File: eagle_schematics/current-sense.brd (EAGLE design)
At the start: 76.2 x 46.7 mm, 19 parts, among them IC1 MCP601P

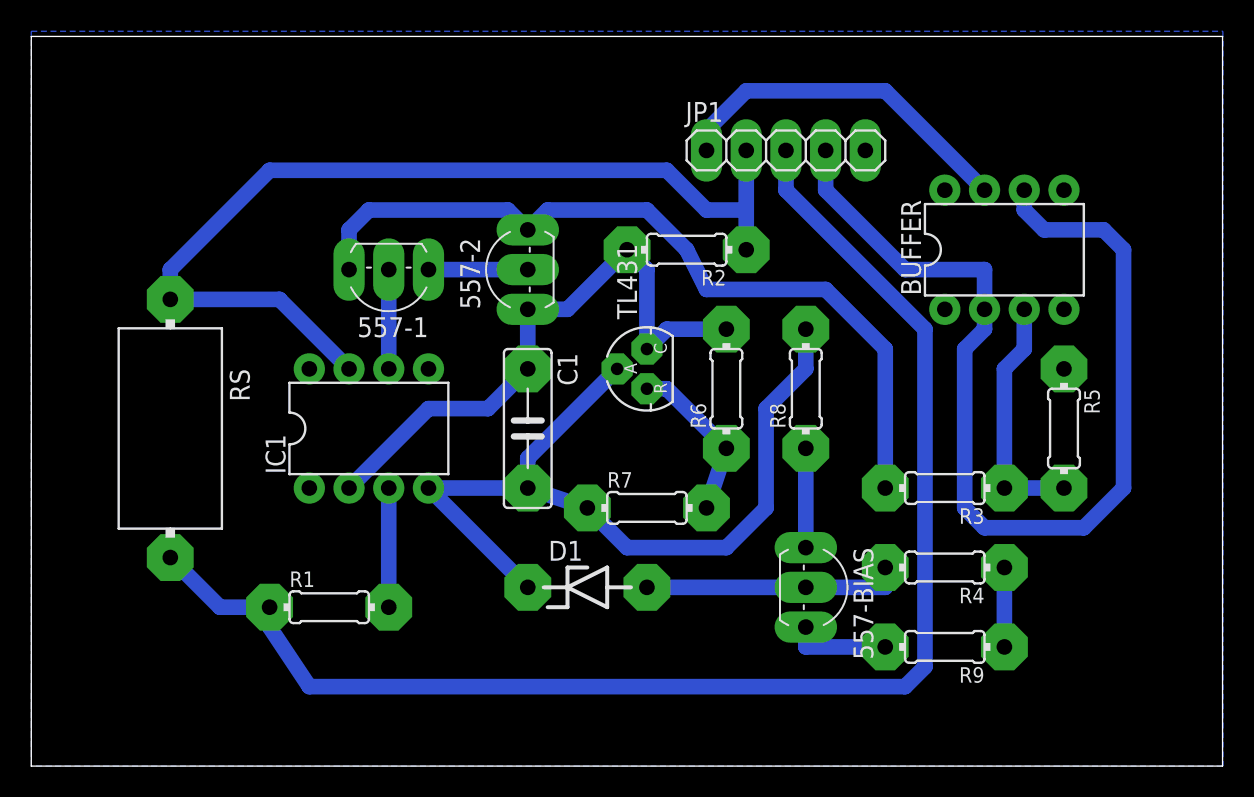
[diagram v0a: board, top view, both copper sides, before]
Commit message: mais esquemáticos
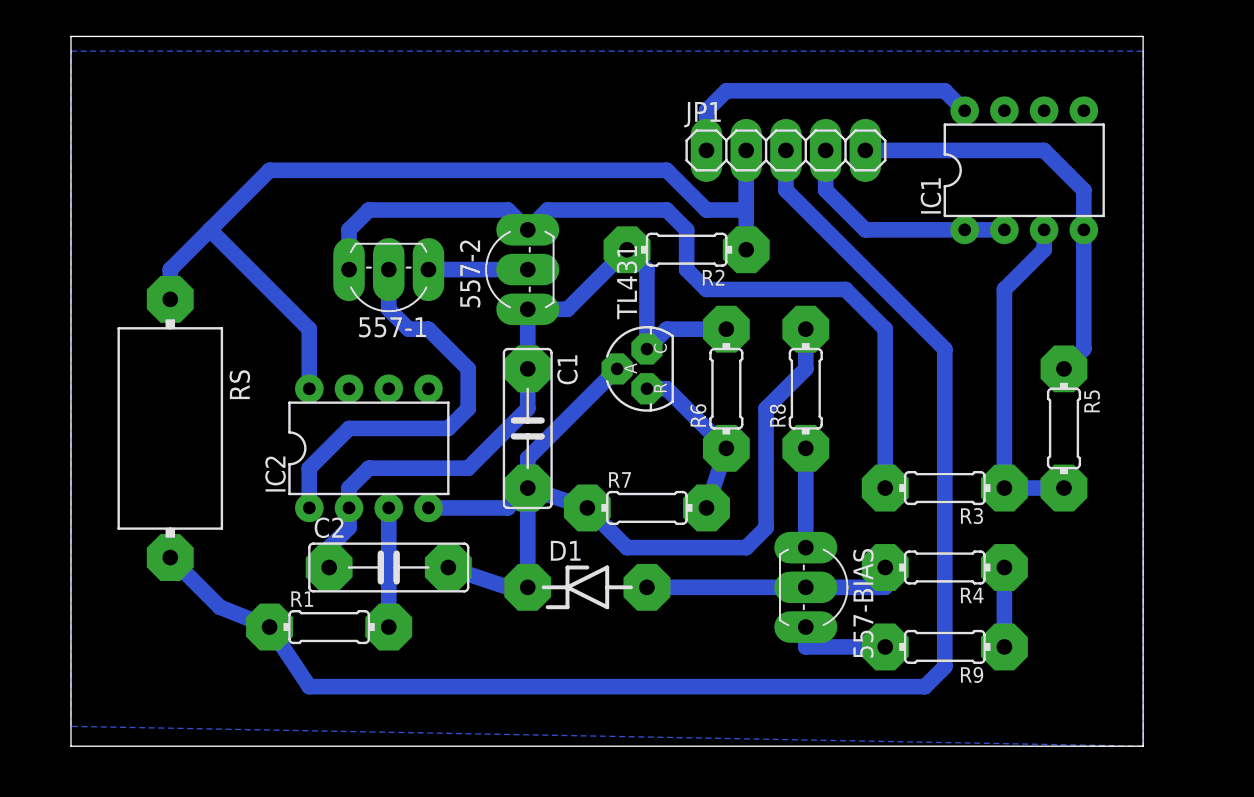
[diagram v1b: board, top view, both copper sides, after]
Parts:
- removed BUFFER: MCP601P, linear:DIL08
- added C2: (no value), rcl:C075-032X103
- added IC2: MCP602P, linear:DIL08
- IC1: value MCP601P -> MCP602P
- R1, R2: value 330 -> 470
- R3: value 6k8 -> 1k
- R4: value 4k7 -> 1k
- R5: value 6k8 -> 8k2
- R6: value 5k6 -> 3k3
- R8: value 180 -> 100
- R9: value 3k9 -> 180
- moved IC1 45.0 mm to (62.2, 35.6)
- moved R1 1.27 mm to (17.8, 6.35)
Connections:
- removed net N$16: C1.2, D1.C, IC1.4, R7.1, R8.2, TL431.A
- removed net N$5: 557-1.B, IC1.6
- new net N$3: 557-1.B, IC2.1
- new net N$4: 557-2.E, C1.1, C2.1, IC2.2, R2.2, R6.2, TL431.C
- net AGND: now also IC1.4; no longer BUFFER.4
- net N$1: now also C1.2, C2.2, D1.C, IC2.4, R7.1, R8.2, TL431.A; no longer 557-2.E, C1.1, IC1.2, R2.2, R6.2, TL431.C
- net N$2: now also IC2.3; no longer IC1.3
- net N$9: now also IC1.3; no longer BUFFER.3
- net OUT: now also IC1.1, IC1.2; no longer BUFFER.2, BUFFER.6
- net SN: now also IC2.8; no longer IC1.7
- net VCC: now also IC1.8; no longer BUFFER.7
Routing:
- net N$16: track 55.3 -> 0.00 mm
- net OUT: track 66.2 -> 15.0 mm
- net N$4: track 0.00 -> 45.9 mm
- net AGND: track 0.00 -> 27.0 mm
- net N$3: track 0.00 -> 26.0 mm
- net N$1: track 38.8 -> 59.3 mm
- net N$5: track 6.35 -> 0.00 mm
- net N$9: track 15.8 -> 21.4 mm
- net VCC: track 22.7 -> 20.1 mm
- net N$10: track 51.5 -> 53.2 mm
- net SP: track 90.1 -> 90.9 mm
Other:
- board size 76.2 x 46.7 mm -> 68.6 x 45.4 mm

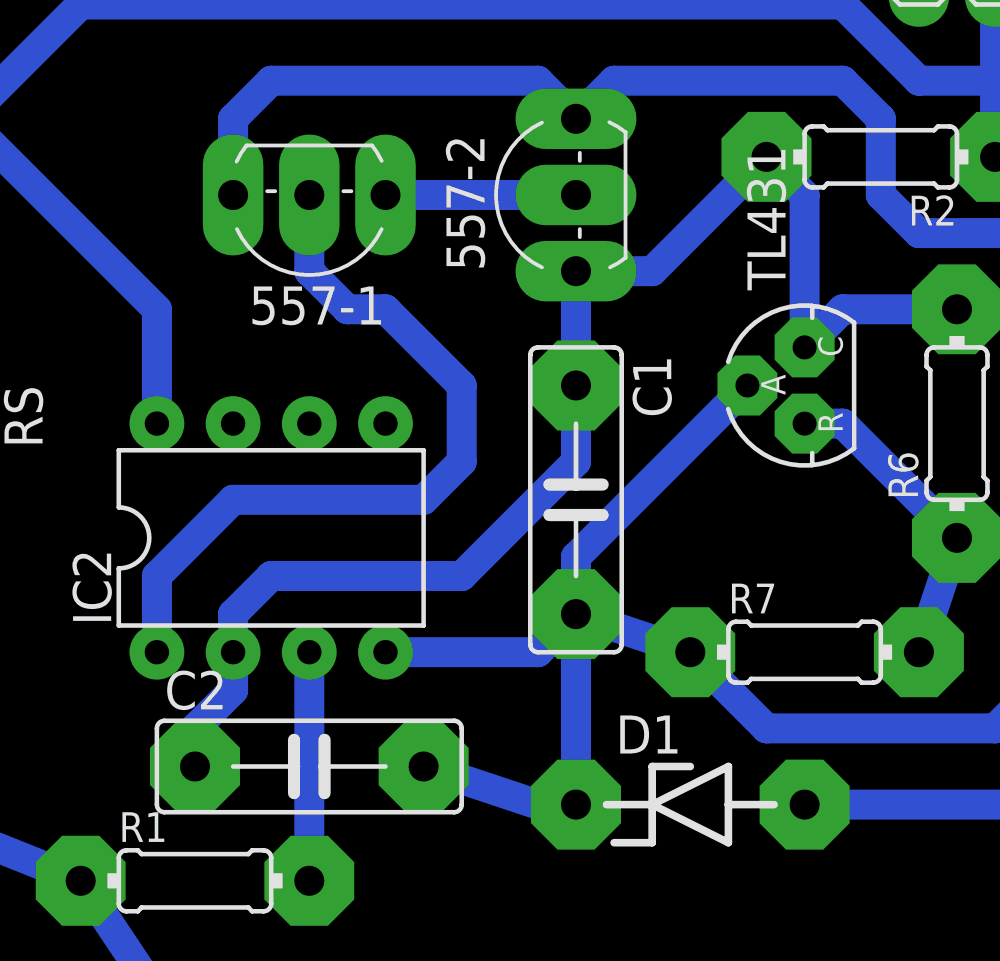
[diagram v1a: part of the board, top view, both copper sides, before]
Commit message: atualizacao de modelos 3D e esquematicos
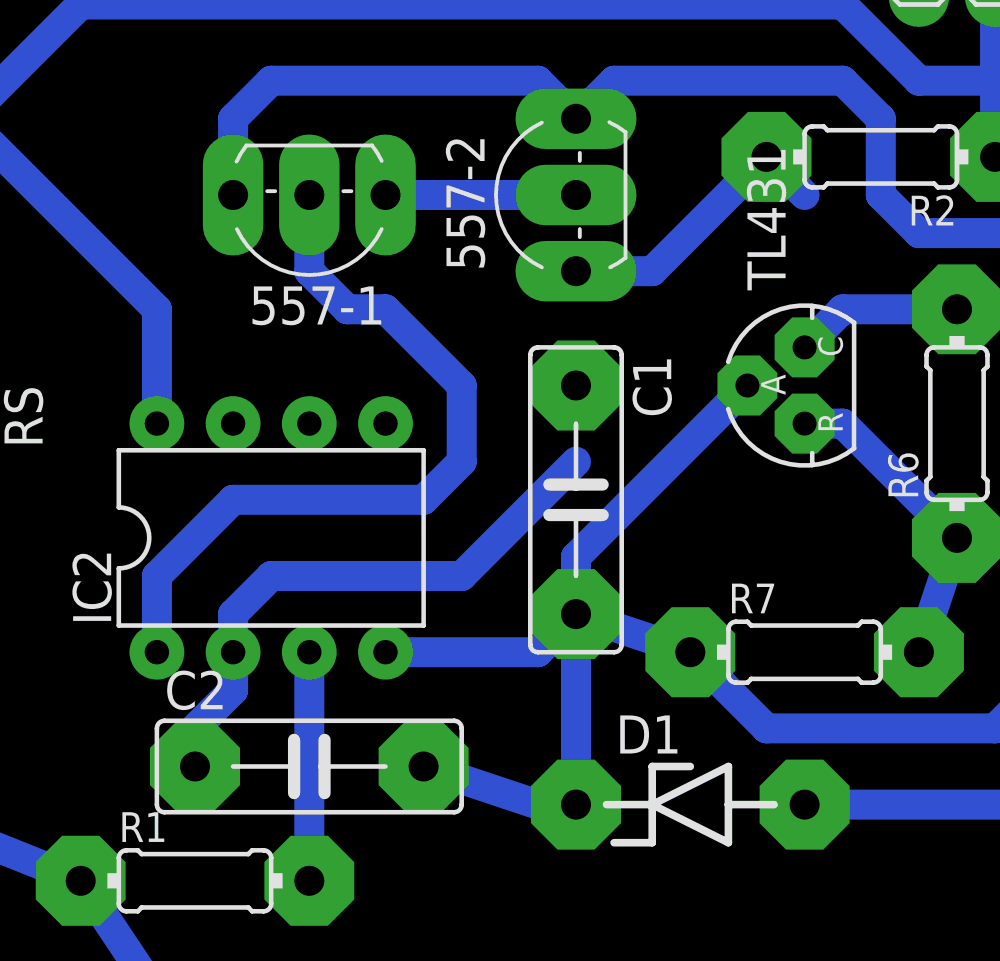
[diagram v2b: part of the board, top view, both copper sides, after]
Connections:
- net N$4: no longer C1.1, C2.1, R6.2, TL431.C
- net SN: now also C1.1, C2.1, R6.2, TL431.C
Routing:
- net N$4: track 45.9 -> 27.6 mm
- net SN: track 61.6 -> 67.2 mm
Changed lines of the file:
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@@
 <?xml version="1.0" encoding="utf-8"?>
 <!DOCTYPE eagle SYSTEM "eagle.dtd">
-<eagle version="7.7.0">
+<eagle version="8.2.1">
 <drawing>
 <settings>
@@
 <wire x1="16.51" y1="21.59" x2="16.51" y2="25.4" width="1" layer="16"/>
 <wire x1="16.51" y1="25.4" x2="10.16" y2="31.75" width="1" layer="16"/>
+<contactref element="C1" pad="1"/>
+<contactref element="R6" pad="2"/>
+<contactref element="TL431" pad="C"/>
+<contactref element="C2" pad="1"/>
+<wire x1="43.18" y1="25.4" x2="39.37" y2="25.4" width="1" layer="16"/>
+<wire x1="39.37" y1="25.4" x2="38.1" y2="24.13" width="1" layer="16"/>
+<wire x1="44.45" y1="30.48" x2="43.18" y2="25.4" width="0" layer="19" extent="1-1"/>
+<wire x1="30.48" y1="22.86" x2="38.1" y2="24.13" width="0" layer="19" extent="1-1"/>
+<wire x1="17.78" y1="10.16" x2="16.51" y2="21.59" width="0" layer="19" extent="1-1"/>
 </signal>
 <signal name="N$6">
@@
 <contactref element="R2" pad="2"/>
 <contactref element="557-2" pad="E"/>
-<contactref element="C1" pad="1"/>
-<contactref element="R6" pad="2"/>
-<contactref element="TL431" pad="C"/>
-<contactref element="C2" pad="1"/>
 <contactref element="IC2" pad="2"/>
-<wire x1="30.48" y1="22.86" x2="30.48" y2="26.67" width="1" layer="16"/>
 <wire x1="30.48" y1="26.67" x2="33.02" y2="26.67" width="1" layer="16"/>
 <wire x1="36.83" y1="30.48" x2="33.02" y2="26.67" width="1" layer="16"/>
-<wire x1="38.1" y1="24.13" x2="38.1" y2="29.21" width="1" layer="16"/>
 <wire x1="38.1" y1="29.21" x2="36.83" y2="30.48" width="1" layer="16"/>
-<wire x1="43.18" y1="25.4" x2="39.37" y2="25.4" width="1" layer="16"/>
-<wire x1="39.37" y1="25.4" x2="38.1" y2="24.13" width="1" layer="16"/>
-<wire x1="17.78" y1="10.16" x2="17.78" y2="11.43" width="1" layer="16"/>
 <wire x1="17.78" y1="11.43" x2="19.05" y2="12.7" width="1" layer="16"/>
 <wire x1="19.05" y1="12.7" x2="19.05" y2="13.97" width="1" layer="16"/>
@@
 <wire x1="20.32" y1="16.51" x2="26.67" y2="16.51" width="1" layer="16"/>
 <wire x1="26.67" y1="16.51" x2="30.48" y2="20.32" width="1" layer="16"/>
-<wire x1="30.48" y1="20.32" x2="30.48" y2="22.86" width="1" layer="16"/>
+<wire x1="30.48" y1="20.32" x2="30.48" y2="26.67" width="0" layer="19" extent="16-16"/>
 </signal>
 </signals>
